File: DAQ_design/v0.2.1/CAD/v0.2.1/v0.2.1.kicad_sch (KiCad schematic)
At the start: 42 parts, among them J1 Screw_Terminal_01x04, U1 Teensy4.0, U2 L293D, U3 PC817, U4 ADS1115IDGS, U5 PC817, U6 PC817, U7 74HC165

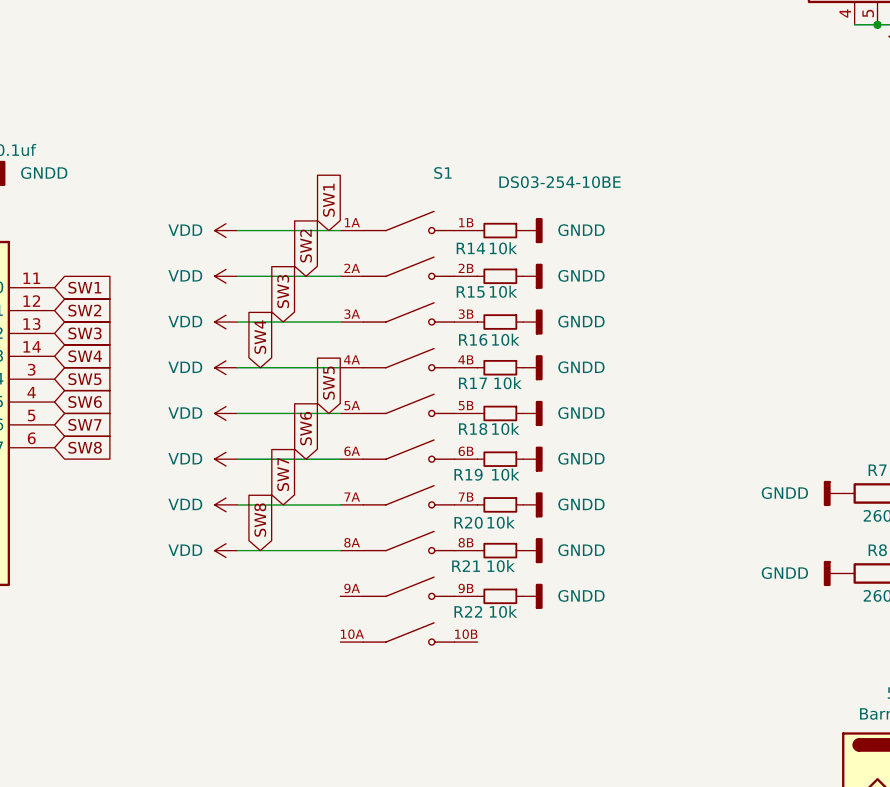
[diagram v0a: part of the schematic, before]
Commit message: routing progress
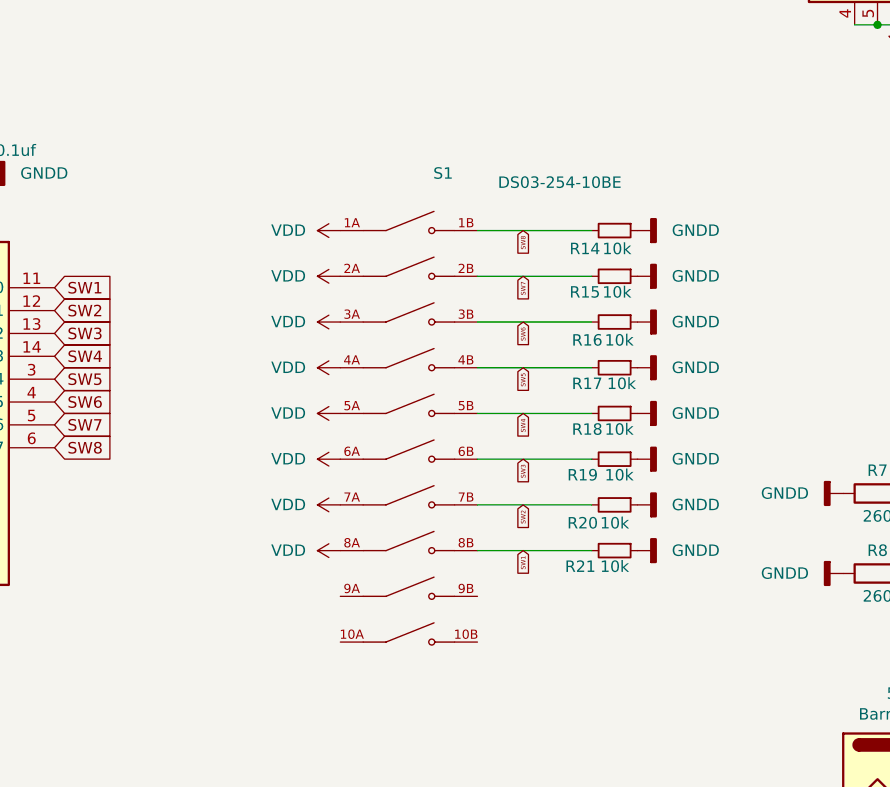
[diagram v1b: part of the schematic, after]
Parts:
- removed R22: 10k, Resistor_SMD:R_1206_3216Metric, symbol Device:R_Small
- R14, R15, R16, R17, R18, R19, R20, R21: footprint Resistor_SMD:R_1206_3216Metric -> Resistor_SMD:R_0805_2012Metric
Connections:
- net VDD: no longer U7.11 (D0), U7.12 (D1), U7.13 (D2), U7.14 (D3), U7.3 (D4), U7.4 (D5), U7.5 (D6), U7.6 (D7)
- net SW6: now reaches R16.2, S1.3B
- net SW6: now also U7.4 (D5)
- net SW4: now reaches R18.2, S1.5B
- net SW4: now also U7.14 (D3)
- net SW1: now reaches R21.2, S1.8B
- net SW1: now also U7.11 (D0)
- net SW5: now reaches R17.2, S1.4B
- net SW5: now also U7.3 (D4)
- net SW2: now reaches R20.2, S1.7B
- net SW2: now also U7.12 (D1)
- net SW8: now reaches R14.2, S1.1B
- net SW8: now also U7.6 (D7)
- net SW7: now reaches R15.2, S1.2B
- net SW7: now also U7.5 (D6)
- net SW3: now reaches R19.2, S1.6B
- net SW3: now also U7.13 (D2)
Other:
- moved on the sheet: R14, R15, R16, R17, R18, R19, R20, R21

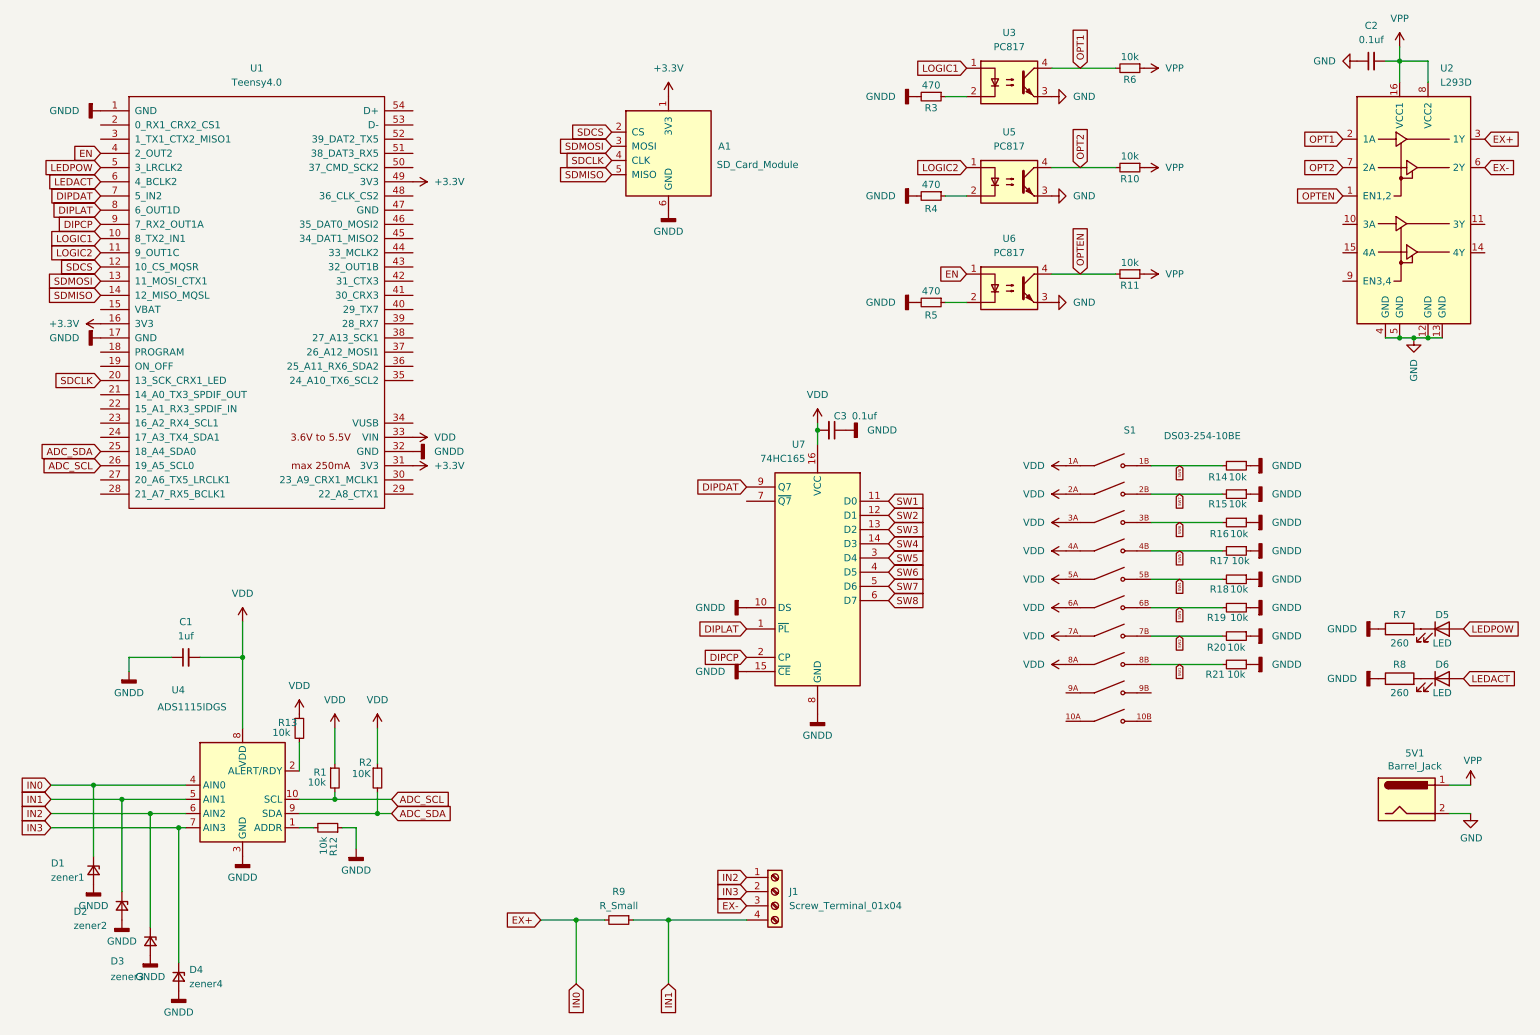
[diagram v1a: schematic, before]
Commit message: update v0.2.1 cad
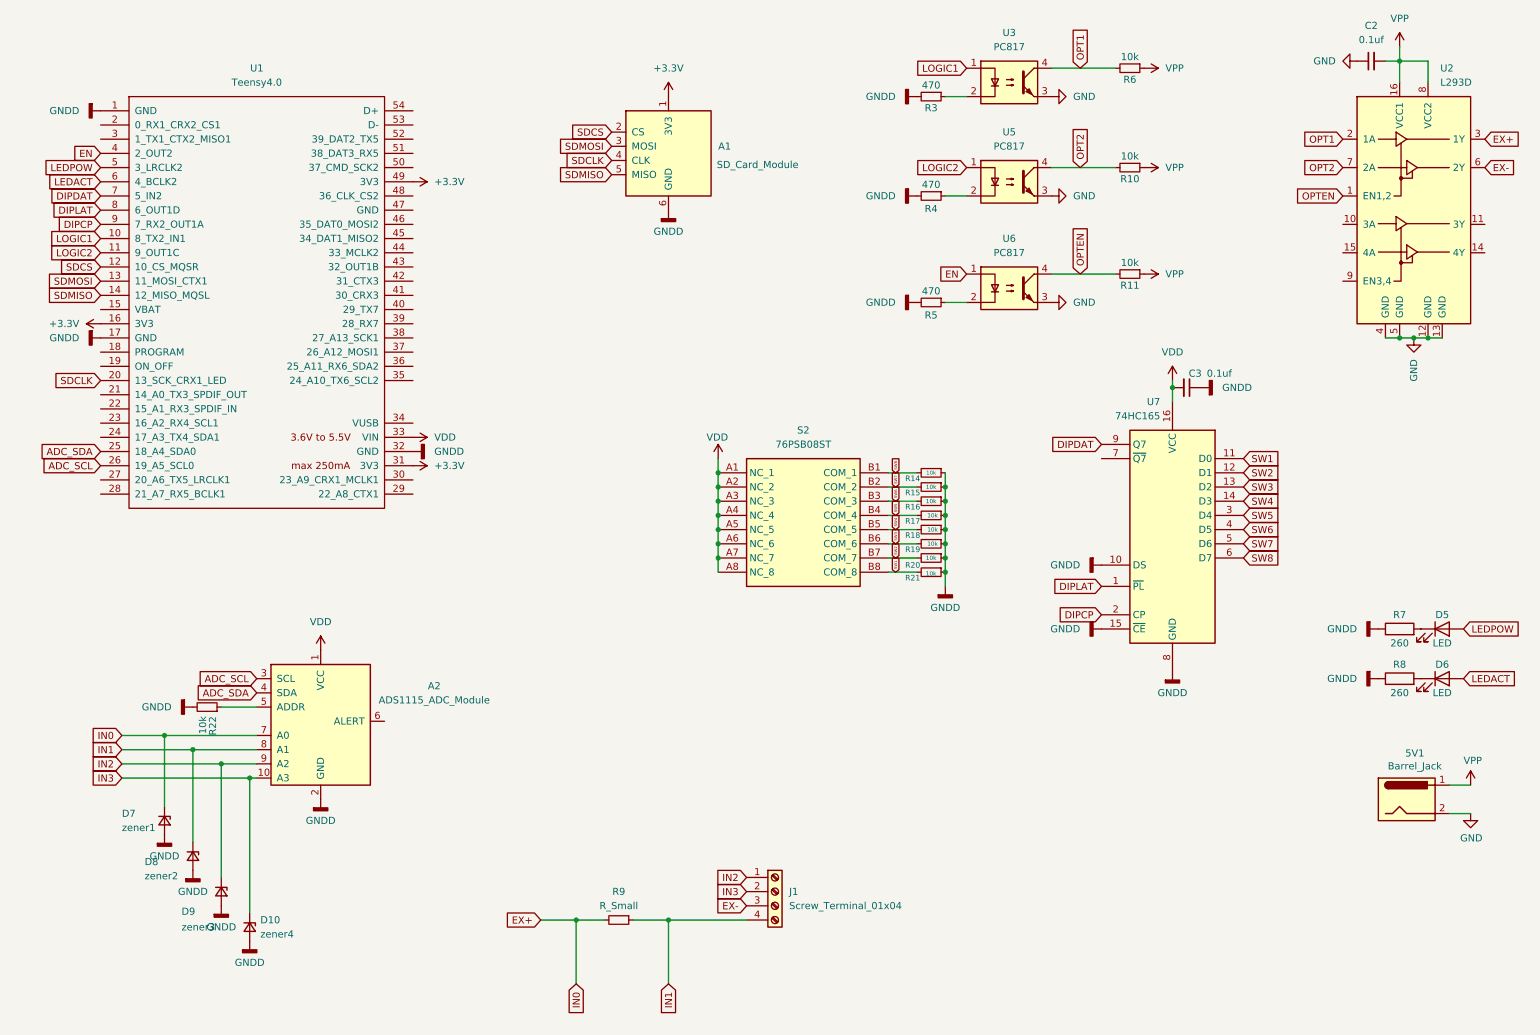
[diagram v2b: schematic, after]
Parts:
- removed C1: 1uf, Capacitor_SMD:C_1206_3216Metric, symbol Device:C_Small
- removed D1: zener1, Diode_THT:D_DO-35_SOD27_P7.62mm_Horizontal, symbol Device:D_Zener_Small
- removed D2: zener2, Diode_THT:D_DO-35_SOD27_P7.62mm_Horizontal, symbol Device:D_Zener_Small
- removed D3: zener3, Diode_THT:D_DO-35_SOD27_P7.62mm_Horizontal, symbol Device:D_Zener_Small
- removed D4: zener4, Diode_THT:D_DO-35_SOD27_P7.62mm_Horizontal, symbol Device:D_Zener_Small
- removed R1, R12, R13: 10k, Resistor_SMD:R_1206_3216Metric, symbol Device:R_Small
- removed R2: 10K, Resistor_SMD:R_1206_3216Metric, symbol Device:R_Small
- removed S1: DS03-254-10BE, dip-switch:SW_DS03-254-10BE, symbol DS03-254-10BE:DS03-254-10BE
- removed U4: ADS1115IDGS, Package_SO:TSSOP-10_3x3mm_P0.5mm, symbol Analog_ADC:ADS1115IDGS
- added A2: ADS1115_ADC_Module, Charleslabs_Parts:ADC1115_ADC_Module, symbol Charleslabs_Parts:ADS1115_ADC_Module
- added D10: zener4, Diode_THT:D_DO-35_SOD27_P7.62mm_Horizontal, symbol Device:D_Zener_Small
- added D7: zener1, Diode_THT:D_DO-35_SOD27_P7.62mm_Horizontal, symbol Device:D_Zener_Small
- added D8: zener2, Diode_THT:D_DO-35_SOD27_P7.62mm_Horizontal, symbol Device:D_Zener_Small
- added D9: zener3, Diode_THT:D_DO-35_SOD27_P7.62mm_Horizontal, symbol Device:D_Zener_Small
- added R22: 10k, Resistor_SMD:R_1206_3216Metric, symbol Device:R_Small
- added S2: 76PSB08ST, 8-pos-dip-switch-foot:76PSB08ST, symbol 8-pos-dip-switch:76PSB08ST
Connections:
- net ADC_SCL: now also A2.3 (SCL)
- net ADC_SDA: now also A2.4 (SDA)
- net EX+: now also A2.7 (A0), D7.1 (K)
- net GNDD: now also A2.2 (GND), D10.2 (A), D7.2 (A), D8.2 (A), D9.2 (A), R22.2
- net IN1: now also A2.8 (A1), D8.1 (K)
- net IN2: now also A2.9 (A2), D9.1 (K)
- net IN3: now also A2.10 (A3), D10.1 (K)
- net SW1: now also S2.B8 (COM_8)
- net SW2: now also S2.B7 (COM_7)
- net SW3: now also S2.B6 (COM_6)
- net SW4: now also S2.B5 (COM_5)
- net SW5: now also S2.B4 (COM_4)
- net SW6: now also S2.B3 (COM_3)
- net SW7: now also S2.B2 (COM_2)
- net SW8: now also S2.B1 (COM_1)
- net VDD: now also A2.1 (VCC), S2.A1 (NC_1), S2.A2 (NC_2), S2.A3 (NC_3), S2.A4 (NC_4), S2.A5 (NC_5), S2.A6 (NC_6), S2.A7 (NC_7), S2.A8 (NC_8)
- new net: A2.5 (ADDR), R22.1
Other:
- moved on the sheet: C3, R14, R15, R16, R17, R18, R19, R20, R21, U7

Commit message: i am a moron
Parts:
- D10, D7, D8, D9: footprint Diode_THT:D_DO-35_SOD27_P7.62mm_Horizontal -> Diode_SMD:D_1206_3216Metric_Pad1.42x1.75mm_HandSolder
- R22: footprint Resistor_SMD:R_1206_3216Metric -> Resistor_SMD:R_0805_2012Metric
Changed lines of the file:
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@@
 			)
 		)
-		(property "Footprint" "Diode_THT:D_DO-35_SOD27_P7.62mm_Horizontal"
+		(property "Footprint" "Diode_SMD:D_1206_3216Metric_Pad1.42x1.75mm_HandSolder"
 			(at 50.8 172.72 90)
 			(effects
@@
 			)
 		)
-		(property "Footprint" "Diode_THT:D_DO-35_SOD27_P7.62mm_Horizontal"
+		(property "Footprint" "Diode_SMD:D_1206_3216Metric_Pad1.42x1.75mm_HandSolder"
 			(at 40.64 160.02 90)
 			(effects
@@
 			)
 		)
-		(property "Footprint" "Diode_THT:D_DO-35_SOD27_P7.62mm_Horizontal"
+		(property "Footprint" "Diode_SMD:D_1206_3216Metric_Pad1.42x1.75mm_HandSolder"
 			(at 45.72 166.37 90)
 			(effects
@@
 			)
 		)
-		(property "Footprint" "Resistor_SMD:R_1206_3216Metric"
+		(property "Footprint" "Resistor_SMD:R_0805_2012Metric"
 			(at 48.26 139.7 0)
 			(effects
@@
 			)
 		)
-		(property "Footprint" "Diode_THT:D_DO-35_SOD27_P7.62mm_Horizontal"
+		(property "Footprint" "Diode_SMD:D_1206_3216Metric_Pad1.42x1.75mm_HandSolder"
 			(at 55.88 179.07 90)
 			(effects
